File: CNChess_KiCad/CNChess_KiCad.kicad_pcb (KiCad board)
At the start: 2 copper layers, 83.5 x 49.1 mm, 32 parts, among them J1 Barrel_Jack, J2 Motor1, J3 Motor2, J4 Servomotor, J5 Fan, SW1 LSW1, SW2 LSW2, SW3 OOSW, U1 ESP32C3, U2 Power_Regulator

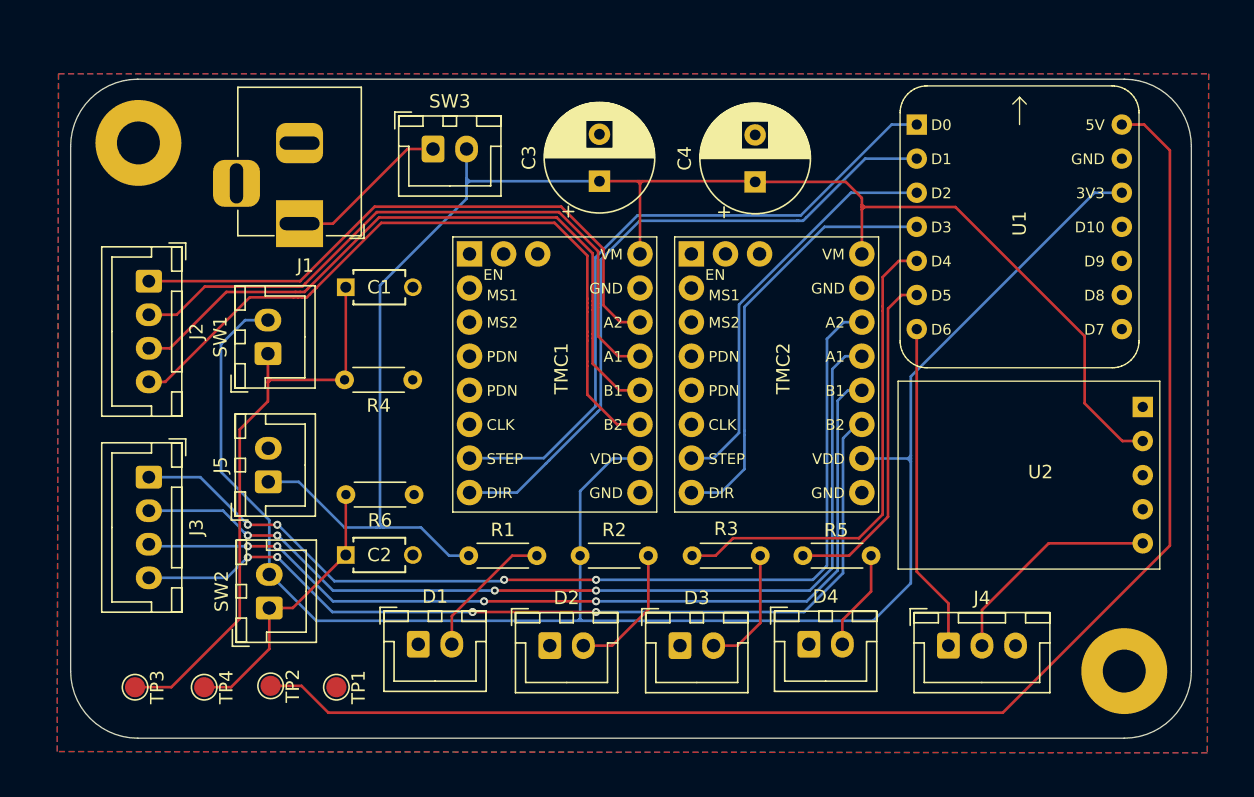
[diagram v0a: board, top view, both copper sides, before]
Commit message: ajout des modèles 3d et terminé V1 du PCB
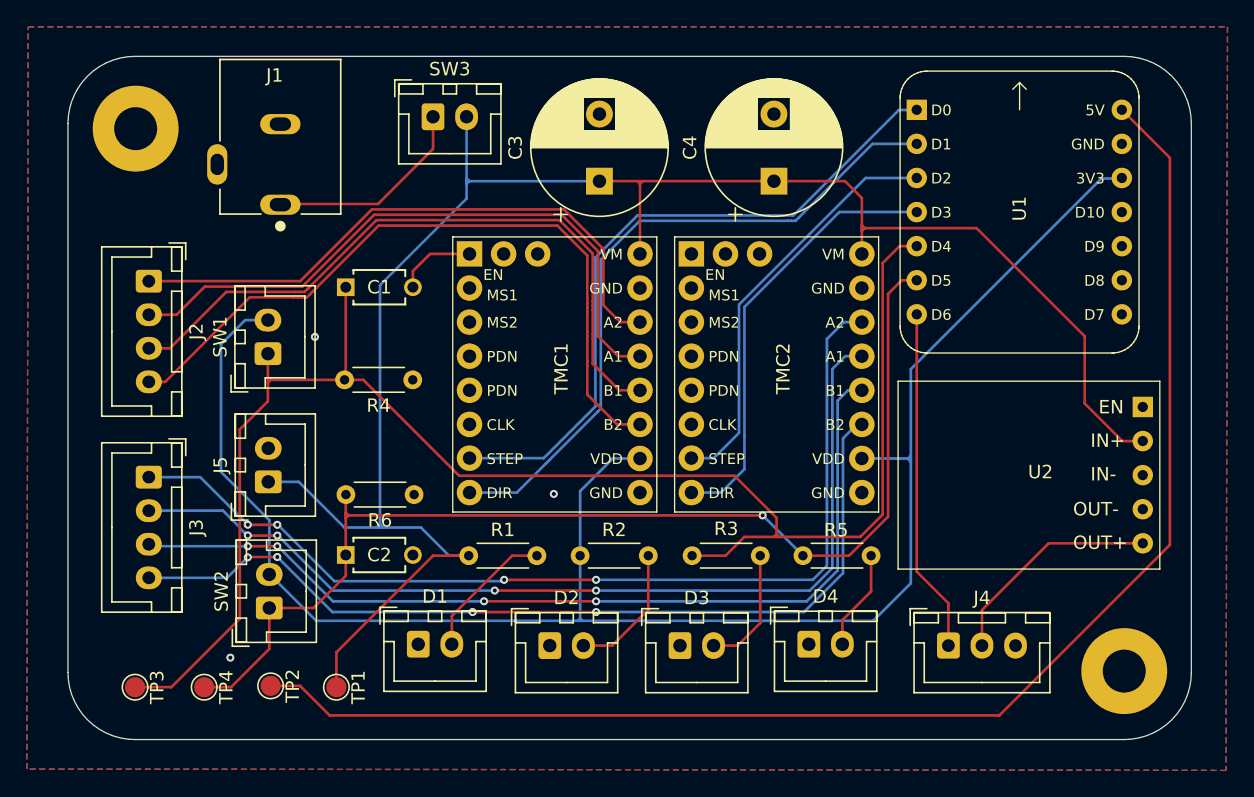
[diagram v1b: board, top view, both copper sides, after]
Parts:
- C3, C4: footprint Capacitor_THT:CP_Radial_D8.0mm_P3.50mm -> Capacitor_THT:CP_Radial_D10.0mm_P5.00mm
- moved J1 8.04 mm to (129.5, 82.3), turned to 90 degrees
- moved SW3 2.40 mm to (140.9, 82.3)
- moved C4 1.40 mm to (166.3, 87.1)
- moved U1 1.10 mm to (184.6, 89.4)
- moved H1 1.08 mm to (118.7, 83.2)
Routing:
- net SW1: track 79.8 -> 119.3 mm
- net SW2: track 46.6 -> 84.5 mm, vias 0 -> 1
- net +12V: track 121.1 -> 138.4 mm
- net GND: track 0.00 -> 5.95 mm, vias 0 -> 3
- net Net-(SW3-A): track 12.7 -> 15.5 mm
- net SERVO: track 24.6 -> 25.7 mm
- net +3V3: track 129.8 -> 130.5 mm
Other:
- board size 83.5 x 49.1 mm -> 83.7 x 50.9 mm
